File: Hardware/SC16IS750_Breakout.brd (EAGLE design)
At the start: 27.9 x 22.9 mm, 17 parts, among them IC1 SC16IS750, Q1 14.7456MHz, U1 3.3V

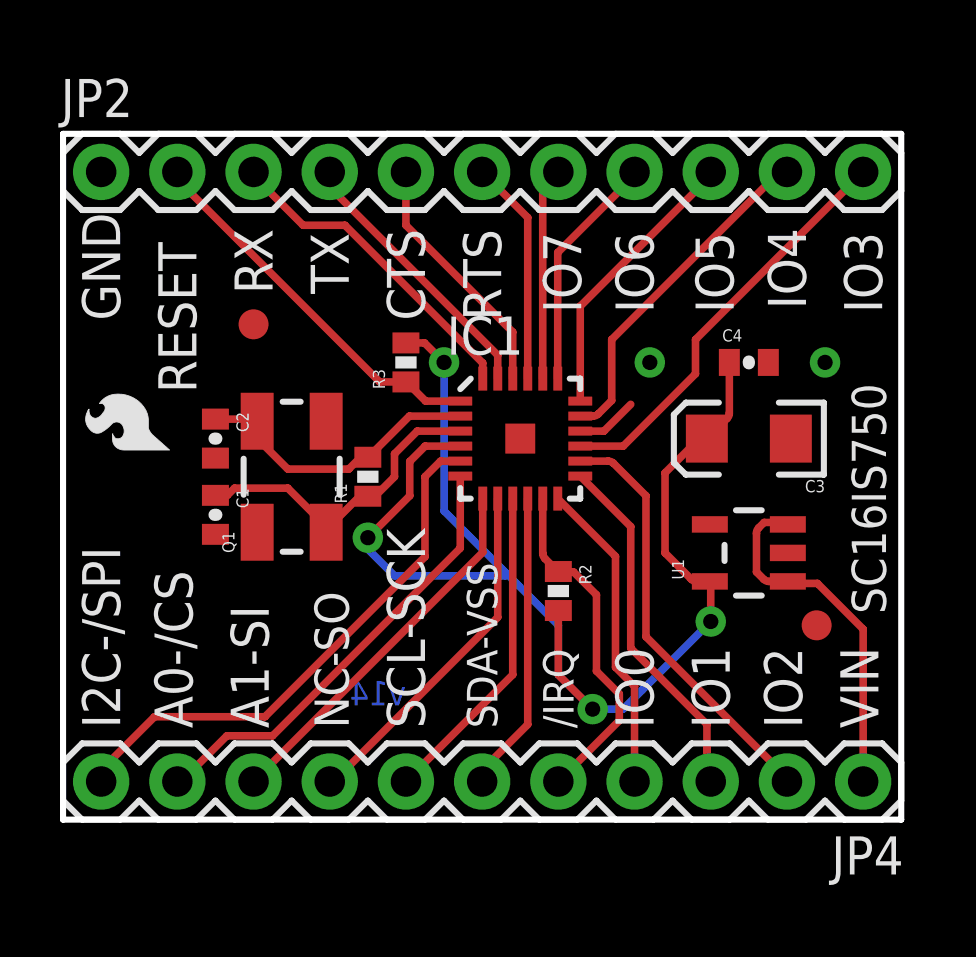
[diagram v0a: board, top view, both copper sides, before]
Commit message: Fixed board files
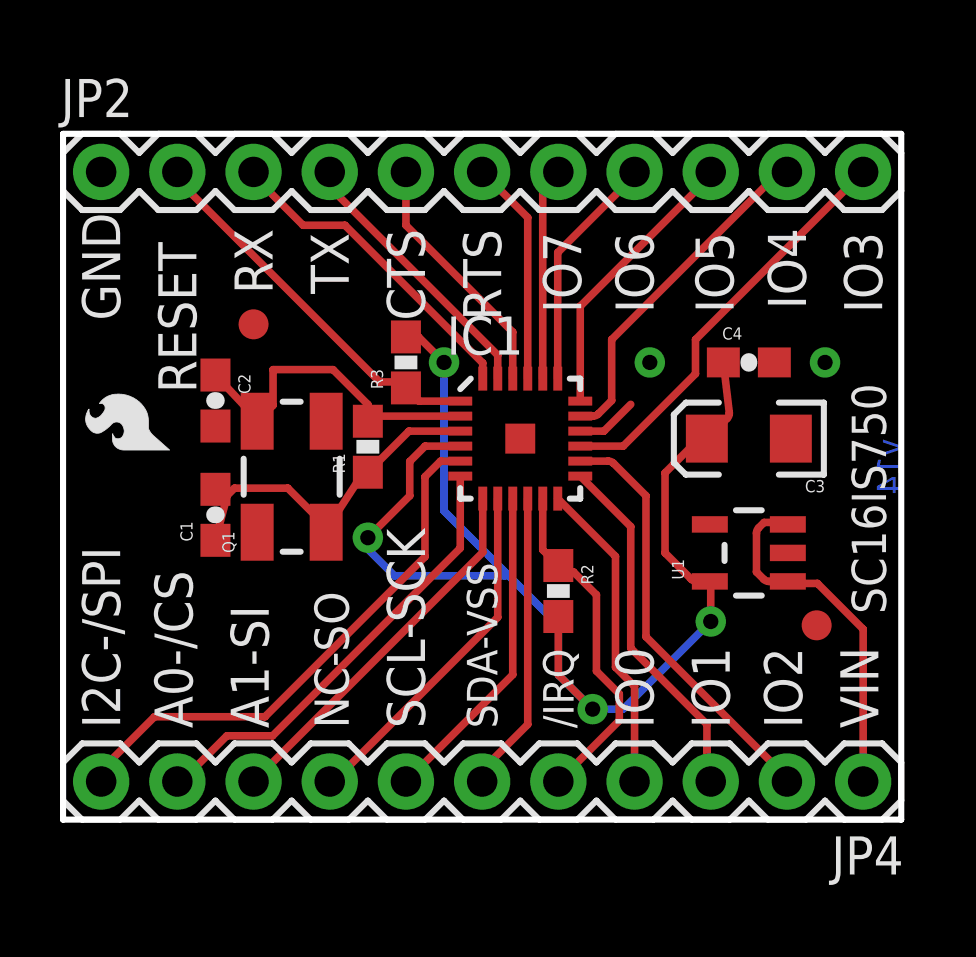
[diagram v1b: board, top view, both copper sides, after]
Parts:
- added U$2: (no value), SparkFun-Aesthetics:CREATIVE_COMMONS
- C1, C2, C4: device SparkFun:0402-CAP -> SparkFun-Passives:0603-CAP
- IC1: device SparkFun:QFN-24 -> SparkFun-DigitalIC:QFN-24
- R1, R2, R3: device SparkFun:0402-RES -> SparkFun-Passives:0603-RES
- moved C2 1.27 mm to (5.08, 14.0)
- moved R1 1.00 mm to (10.2, 12.4)
- turned C1 to 90 degrees
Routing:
- net N$24: track 9.98 -> 12.3 mm
- net N$23: track 11.0 -> 12.4 mm
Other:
- board text added: "C. Taylor, Updated by: T. Klopfenstein"
